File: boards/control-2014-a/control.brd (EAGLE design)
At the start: 285 parts, among them J1 0528520870, J10 2MM-6H, J11 JST_VH_2, J12 2MM-4V, J13 2MM-4H, J14 2MM-4H, J15 2MM-4H, J16 2MM-4H, J17 2MM-8H, J19 JST_VH_2, J2 MINI-USB, J20 2MM-5V, J3 2MM-2H, J4 Molex 0522711179, J5 Molex 0522711179, J6 Molex 0522711179, J7 Molex 0522711179, J8 MMCX_RA, J9 2MM-3H, Q1 IRF9310TRPBF, Q10 IRF8734TRPBF, Q11 IRF9310TRPBF, Q12 IRF8734TRPBF, Q13 IRF9310TRPBF, Q14 IRF8734TRPBF, Q15 IRF9310TRPBF, Q16 IRF8734TRPBF, Q17 IRF9310TRPBF, Q18 IRF8734TRPBF, Q19 IRF9310TRPBF, Q2 IRF8734TRPBF, Q20 IRF8734TRPBF, Q21 IRF9310TRPBF, Q22 IRF8734TRPBF, Q23 IRF9310TRPBF, Q24 IRF8734TRPBF, Q25 IRF9310TRPBF, Q26 IRF8734TRPBF, Q27 IRF9310TRPBF, Q28 IRF8734TRPBF, Q29 IRF9310TRPBF, Q3 IRF9310TRPBF, Q30 IRF8734TRPBF, Q33 FDV304P, Q4 IRF8734TRPBF, Q5 IRF9310TRPBF, Q6 IRF8734TRPBF, Q7 IRF9310TRPBF, Q8 IRF8734TRPBF, Q9 IRF9310TRPBF, U1 XC3S100E, U10 CC1101, U12 TC4428, U13 0896BM15A0001, U15 TC4428, U18 TC4428, U19 IMU3000, U2 M25P10, U20 KXTF9-2050, U21 TC4428, U24 TC4428, U27 TC4428, U3 LM2734, U30 TC4428, U33 TC4428, U36 TC4428, U39 TC4428, U4 MCP1824T-1202E/OT, U42 TC4428, U45 TC4428, U48 TC4428, U5 MCP1824T-2502E/OT, U6 TC4428, U7 AT91SAM7S256, U8 MCP1824ST-3302E/DB, U9 TC4428, X1 18.432MHz, X2 644-1055-1-ND

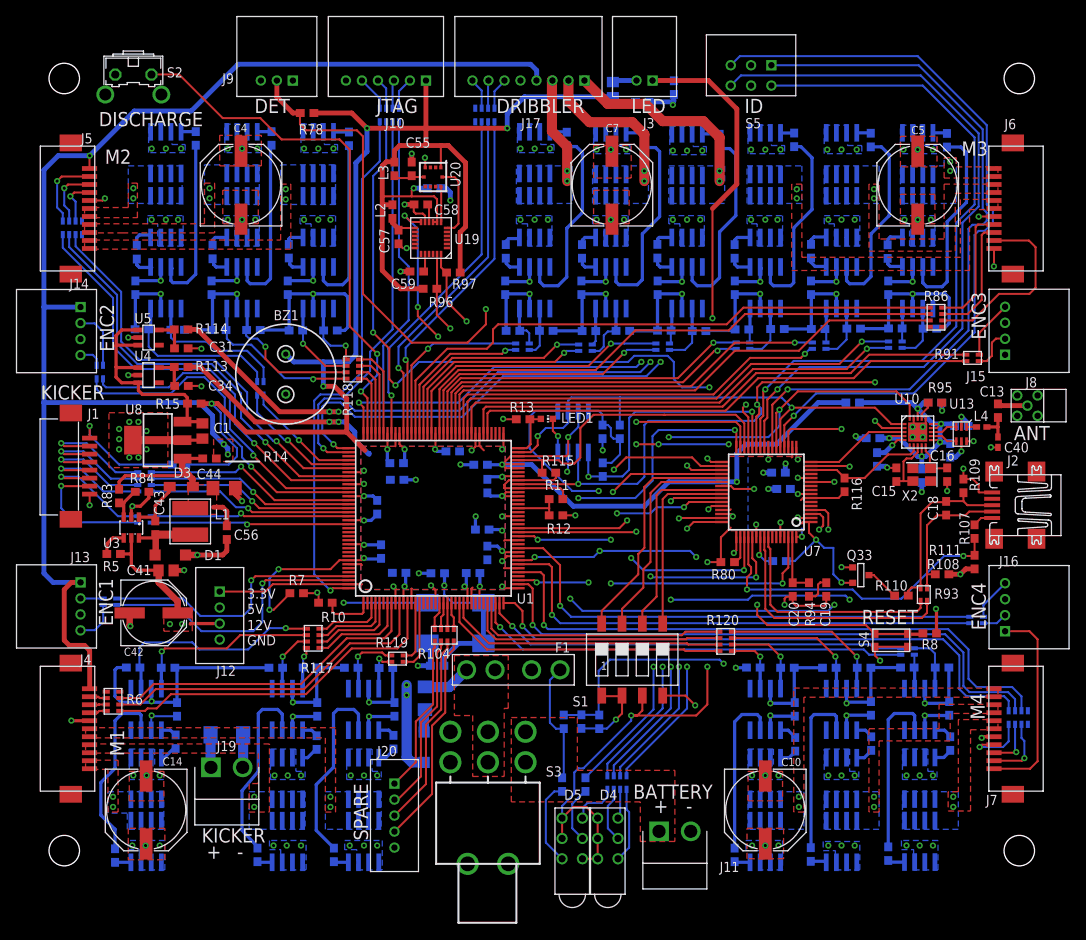
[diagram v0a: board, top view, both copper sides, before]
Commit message: control-2014-a
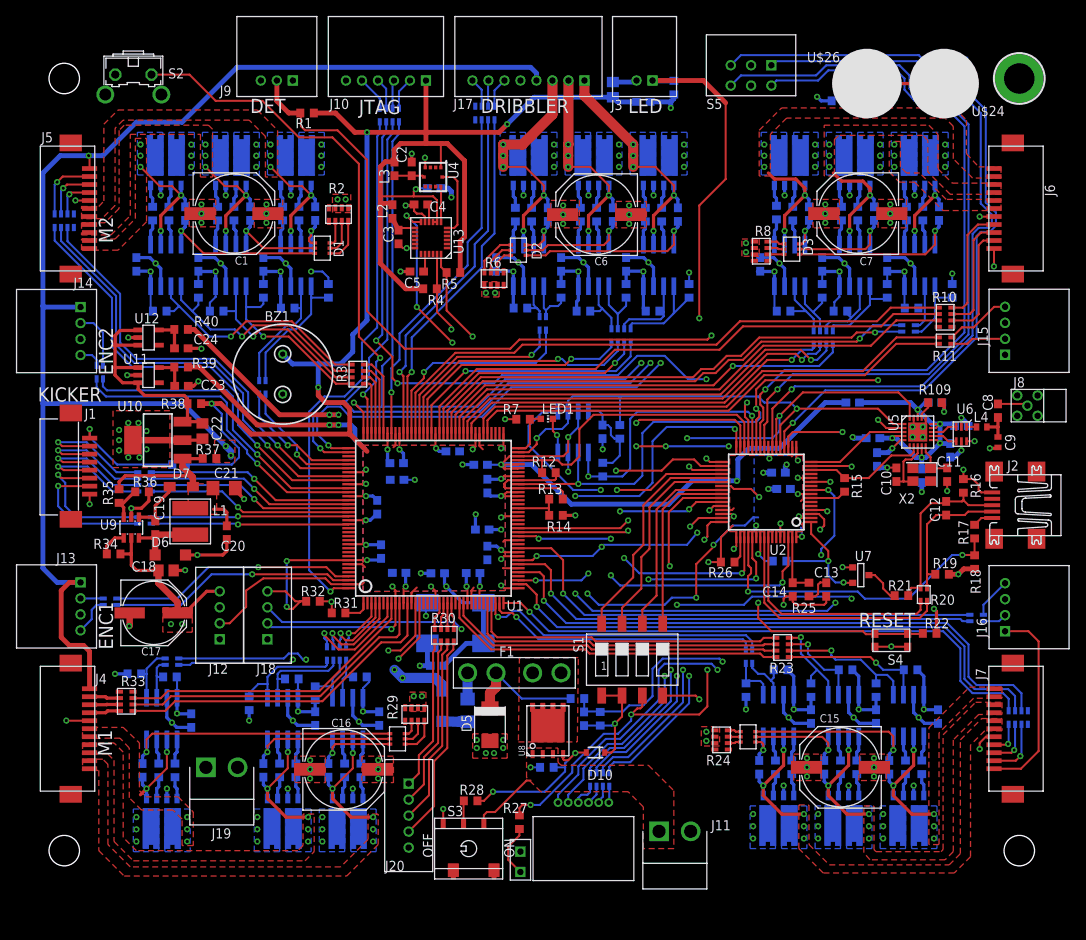
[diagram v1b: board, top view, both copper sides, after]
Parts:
- removed Q33: FDV304P, zetex:SOT-23
- removed R131: 220, resistor-array:RA_2_0606
- removed U15, U18, U21, U24, U27, U30, U33, U36, U39, U42, U45, U48: TC4428, microchip:SO08
- removed U19: IMU3000, inertial-sensors:IMU3000
- removed U20: KXTF9-2050, inertial-sensors:KXTF9
- added C45, C69, C75: 47nF, rcl:C0603
- added C61, C63, C64, C65, C66, C70, C72, C73, C74, C76, C78: 100nF, rcl:C0603
- added C62: 10nF, rcl:C0603
- added D10: CDSOD323-T15SC, CDSOD323-TxxSC:SOD-323
- added D7: BAS16H, diode:SOD323-W
- added D8: MMBD4448HTW, Diode-Array:MMBD4448HTW
- added D9: MBRX160-TP, diode:SOD123
- added H1: (no value), Mounting_Hole:MOUNTING_HOLE
- added J18: 2MM-4V, 2mm:2MM-4-V
- added LED2: LED2, 5350T5:5350T5
- added LED3: LDS-M514RI-RA, rjrc-7seg-disp:LDS-M514RI-RA
- added R100: 220, resistor-array:RA_2_0606
- added R101, R121: 10.0k, rcl:R0603
- added R106, R126: 220, resistor-array:RA_4_1206
- added R127: 0, rcl:R0603
- added R98, R99: 22, rcl:R0603
- added U$24, U$26: RL1014, RLB1014-inductor:RL1014
- added U11: MCP1824T-1202E/OT, power:SOT23-5
- C1: value 10uF -> 470uF 25V; device rcl:C0805 -> rcl:PANASONIC_G
- C10: value 470uF 25V -> 27pF; device rcl:PANASONIC_G -> rcl:C0603
- C11: value 10nF -> 27pF
- C12: value 220nF -> 33pF
- C13: value 100pF -> 10nF
- C14: value 470uF 25V -> 1nF; device rcl:PANASONIC_G -> rcl:C0603
- C15, C16: value 27pF -> 470uF 25V; device rcl:C0603 -> rcl:PANASONIC_G
- C17: value 100nF -> 100uF 25V; device rcl:C0603 -> rcl:PANASONIC_E
- C18: value 33pF -> 1uF 35V; device rcl:C0603 -> rcl:C0805
- C20: value 1nF -> 100nF
- C21: value 100nF -> 22uF 6.3V; device rcl:C0603 -> rcl:C1206
- C22: value 100nF -> 10uF; device rcl:C0603 -> rcl:C0805
- C23, C24, C50: value 100nF -> 1uF
- C3, C31, C34: value 1uF -> 100nF
- C38, C47, C49, C52, C54, C56, C67, C71, C77, C79: value 100nF -> 47nF
- C4: value 470uF 25V -> 100nF; device rcl:PANASONIC_G -> rcl:C0603
- C40: value 500R07S1R8BV4T -> 47nF; device rcl:C0402 -> rcl:C0603
- C41: value 1uF 35V -> 100nF; device rcl:C0805 -> rcl:C0603
- C42: value 100uF 25V -> 47nF; device rcl:PANASONIC_E -> rcl:C0603
- C43: value 10nF -> 100nF
- C44: value 22uF 6.3V -> 100nF; device rcl:C1206 -> rcl:C0603
- C5: value 470uF 25V -> 2.2nF; device rcl:PANASONIC_G -> rcl:C0603
- C57: value 100nF -> 220nF
- C6: value 100nF -> 470uF 25V; device rcl:C0603 -> rcl:PANASONIC_G
- C60: value 100nF -> 10nF
- C8: value 10nF -> 100pF
- C9: value 2.2nF -> 500R07S1R8BV4T; device rcl:C0603 -> rcl:C0402
- D1, D2: value MBRX160-TP -> MMBD4448HTW; device diode:SOD123 -> Diode-Array:MMBD4448HTW
- D3: value BAS16H -> MMBD4448HTW; device diode:SOD323-W -> Diode-Array:MMBD4448HTW
- D4: value 564-0100-132F -> MMBD4448HTW; device led-array:DIALIGHT-564 -> Diode-Array:MMBD4448HTW
- D5: value 564-0100-132F -> SMBJP6KE18A-TP; device led-array:DIALIGHT-564 -> power:SMBJ
- D6: value SMBJP6KE18A-TP -> MBRX160-TP; device power:SMBJ -> diode:SOD123
- F1: value 2x BK6011 -> 2x BK6011 [30A]
- J11: value JST_VH_2 -> BATT
- Q1, Q11, Q13, Q15, Q17, Q19, Q21, Q23, Q25, Q27, Q29, Q3, Q5, Q7, Q9: value IRF9310TRPBF -> FAN7380; device onsemi:SO8 -> microchip:SO08
- Q10, Q12, Q14, Q16, Q18, Q2, Q20, Q22, Q24, Q26, Q28, Q30, Q4, Q6, Q8: value IRF8734TRPBF -> BSC072N03LD; device onsemi:SO8 -> Dual N-Channel MOSFET:BSC072N03LD
- R1: value 220 -> 5.6k; device resistor-array:RA_4_1206 -> rcl:R0603
- R10: device rcl:R0603 -> resistor-array:RA_4_1206
- R102, R14, R15: value 0 -> 10.0k
- R103, R122, R123: value 220 -> 22; device resistor-array:RA_2_0606 -> rcl:R0603
- R104, R117, R118, R85, R86: value 220 -> 22; device resistor-array:RA_4_1206 -> rcl:R0603
- R105: value NP -> 100k
- R107, R79: value 220 -> 10.0k
- R108: value 330k -> 68k
- R109: value 330k -> 56k
- R11: value NP -> 220; device rcl:R0603 -> resistor-array:RA_2_0606
- R110: value 1.5k -> 220; device rcl:R0603 -> resistor-array:RA_4_1206
- R113, R114: value 0 -> 22
- R115: value NP -> 10.0k
- R12: value 10.0k -> NP
- R120, R4, R87, R88: value 220 -> 10.0k; device resistor-array:RA_4_1206 -> rcl:R0603
- R129, R130: value 220 -> 10K; device resistor-array:RA_2_0606 -> rcl:R0603
- R13: value 220 -> NP
- R16: value 100k -> 330k
- R17: value 1.5k -> 220
- R18, R22, R34, R42, R43, R46, R47, R50, R51, R58, R59, R63, R67, R74, R75: value 10 -> 10.0k
- R19: value 10 -> 330k
- R2, R24, R29, R8: value 10.0k -> 22; device rcl:R0603 -> resistor-array:RA_4_1206
- R20: value 10.0k -> 27; device rcl:R0603 -> resistor-array:RA_2_0606
- R21, R25: value 10.0k -> 1.5k
- R23, R30, R55, R62: value 10 -> 220; device rcl:R0603 -> resistor-array:RA_4_1206
- R26: value 10 -> NP
- R27, R31: value 10 -> 220
- R28: value 10.0k -> 10
- R33, R41, R56, R73: value 10.0k -> 220; device rcl:R0603 -> resistor-array:RA_4_1206
- R35: value 10 -> 52.3k
- R37, R40: value 10.0k -> 0
- R38, R39: value 10 -> 0
- R44, R45, R48, R49, R52, R53, R60, R61, R65, R69, R76, R77: value 10.0k -> 22
- R54: value 10 -> 220; device rcl:R0603 -> resistor-array:RA_2_0606
- R57, R82: value 10.0k -> 220; device rcl:R0603 -> resistor-array:RA_2_0606
- R6: value 220 -> 22
- R66, R70: value 10 -> 22
- R7: value 10.0k -> 220
- R71: value 10 -> 150 1/8W; device rcl:R0603 -> rcl:R0805
- R72: value 10.0k -> 100k
- R78: value 5.6k -> 10.0k
- R80: value NP -> 22
- R81: value 68k -> 22
- R83: value 52.3k -> 10.0k
- R89: value 220 -> NP; device resistor-array:RA_2_0606 -> rcl:R0603
- R9: value 150 1/8W -> 10K; device rcl:R0805 -> rcl:R0603
- R91: device resistor-array:RA_2_0606 -> resistor-array:RA_4_1206
- R92: value 220 -> 10.0k; device resistor-array:RA_2_0606 -> rcl:R0603
- R93: value 27 -> 10.0k; device resistor-array:RA_2_0606 -> rcl:R0603
- R94: value 1.5k -> 22
- R95: value 56k -> 22
- S3: value M2022S2A2W30 -> G3T12AP_SPDT; device switch-robocup:M202X-30 -> switch-robocup:G3T12AP_SP
- U10: value CC1101 -> MCP1824ST-3302E/DB; device radio:QLP20 -> power:SOT223
- U12: value TC4428 -> MCP1824T-2502E/OT; device microchip:SO08 -> power:SOT23-5
- U13: value 0896BM15A0001 -> IMU3000; device radio:0896BM15A0001 -> inertial-sensors:IMU3000
- U2: value M25P10 -> AT91SAM7S256; device st_micro:SO08 -> at91sam7:SQFP-S-10X10-64
- U3: value LM2734 -> M25P10; device power:SOT23-6L -> st_micro:SO08
- U4: value MCP1824T-1202E/OT -> KXTF9-2050; device power:SOT23-5 -> inertial-sensors:KXTF9
- U5: value MCP1824T-2502E/OT -> CC1101; device power:SOT23-5 -> radio:QLP20
- U6: value TC4428 -> 0896BM15A0001; device microchip:SO08 -> radio:0896BM15A0001
- U7: value AT91SAM7S256 -> FDV304P; device at91sam7:SQFP-S-10X10-64 -> zetex:SOT-23
- U8: value MCP1824ST-3302E/DB -> SI7141DP; device power:SOT223 -> rjrc_power_transistors:POWERPAK_SO-8
- U9: value TC4428 -> LM2734; device microchip:SO08 -> power:SOT23-6L
- moved Q8 121.7 mm to (12.7, 86.0), turned to 90 degrees
- moved Q6 121.0 mm to (12.2, 3.68), turned to 270 degrees
- moved R90 113.8 mm to (114.0, 29.1), turned to 90 degrees
- moved Q24 107.3 mm to (89.3, 4.06), turned to 270 degrees
- moved R128 106.8 mm to (4.45, 59.8), turned to 0 degrees
- moved R123 106.3 mm to (11.8, 10.0), turned to 270 degrees
- moved R22 105.5 mm to (108.2, 27.2), flipped to the top, turned to 0 degrees
- moved R55 105.3 mm to (40.6, 91.9), turned to 0 degrees
- moved R84 104.3 mm to (111.0, 70.0), flipped to the bottom, turned to 270 degrees
- moved R85 104.3 mm to (105.3, 79.6), turned to 90 degrees
- moved Q23 104.0 mm to (89.3, 16.9)
- moved R83 101.8 mm to (105.9, 67.8), flipped to the bottom, turned to 180 degrees
- moved R42 100.7 mm to (11.9, 67.4), turned to 180 degrees
- moved R44 98.2 mm to (11.0, 79.6), turned to 90 degrees
- moved C18 97.8 mm to (12.7, 35.0), turned to 0 degrees
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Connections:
- removed net LED_LR: R1.8, U7.35
- removed net LED_LY: R79.1, U7.42
- removed net LED_RG: R1.2, U7.48
- removed net LED_RR: R1.4, U7.47
- removed net LED_RY: R1.6, U7.15
- new net CHASSIS: H1.GND, R9.1, U$24.P$1
- new net LED_AE: R106.8, U2.35
- new net LED_AN1: LED3.1, U2.9
- new net LED_AN2: LED3.2, U2.42
- new net LED_BF: R106.6, U2.15
- new net LED_CG: R106.4, U2.47
- new net LED_DDP: R106.2, U2.48
- new net N$100: Q17.7, R86.1
- new net N$174: Q11.2, R62.4, R67.2
- new net N$175: Q11.7, R70.1
- new net N$176: D2.A2, R6.5
- new net N$177: Q26.G1, R70.2
- new net N$178: Q11.5, R69.1
- new net N$179: Q26.G2, R69.2
- new net N$180: Q11.1, R62.2, R68.2
- new net N$181: Q9.2, R62.8, R63.2
- new net N$182: Q9.7, R66.1
- new net N$183: Q28.G1, R66.2
- new net N$184: Q9.5, R65.1
- new net N$185: Q28.G2, R65.2
- new net N$186: Q9.1, R62.6, R64.2
- new net N$187: Q7.2, R57.4, R58.2
- new net N$188: Q7.7, R61.1
- new net N$189: Q30.G1, R61.2
- new net N$190: Q7.5, R60.1
- new net N$191: Q30.G2, R60.2
- new net N$192: Q7.1, R57.2, R59.2
- new net N$193: C49.1, D2.C3, Q11.8
- new net N$194: C47.1, D2.C2, Q9.8
- new net N$195: C45.1, D2.C1, Q7.8
- new net N$196: D2.A1, R6.7
- new net N$197: D2.A3, R6.3
- new net N$198: R28.1, S3.5
- new net N$199: D10.2, R105.1, R28.2, U8.4
- new net N$200: R130.2, U$24.P$2, U$26.P$1
- new net N$201: R129.1, U$26.P$2
- new net N$3: Q25.2, R110.8, R111.2
- new net N$94: F1.1, F1.2, U8.D@1, U8.D@2, U8.D@3, U8.D@4
- new net N$95: Q15.1, R73.2, R79.2
- new net VBATT: J11.1, R105.2, S3.4, U8.S@1, U8.S@2, U8.S@3
- net +1.2V: now also C26.1, C27.1, C31.1, C34.1, J18.2, R39.1; no longer C24.1, C50.1, C51.1, C71.1, R113.1
- net +1.8V: now also C64.1, J18.3, U2.12, U2.24, U2.54, U2.64, U2.8; no longer C79.1, U7.12, U7.24, U7.54, U7.64, U7.8
- net +12V: now also C1.+, C15.+, C16.+, C41.1, C44.1, C46.1, C48.1, C51.1, C53.1, C55.1, C6.+, C66.1, C68.1, C70.1, C74.1, C76.1, C78.1, D5.C, F2.1, Q10.D1@1, Q10.D1@2, Q12.D1@1, Q12.D1@2, Q14.D1@1, Q14.D1@2, Q16.D1@1, Q16.D1@2, Q18.D1@1, Q18.D1@2, Q2.D1@1, Q2.D1@2, Q20.D1@1, Q20.D1@2, Q22.D1@1, Q22.D1@2, Q24.D1@1, Q24.D1@2, Q26.D1@1, Q26.D1@2, Q28.D1@1, Q28.D1@2, Q30.D1@1, Q30.D1@2, Q4.D1@1, Q4.D1@2, Q6.D1@1, Q6.D1@2, Q8.D1@1, Q8.D1@2, R108.2, R2.4, R2.6, R2.8, R24.4, R24.6, R24.8, R29.4, R29.6, R29.8, R6.4, R6.6, R6.8, R8.4, R8.6, R8.8; no longer C10.+, C14.+, C2.1, C21.1, C22.1, C26.1, C27.1, C28.1, C29.1, C30.1, C32.1, C33.1, C35.1, C36.1, C38.1, C4.+, C5.+, D6.C, Q1.1, Q1.2, Q11.1, Q11.2, Q13.1, Q13.2, Q15.1, Q15.2, Q17.1, Q17.2, Q19.1, Q19.2, Q21.1, Q21.2, Q23.1, Q23.2, Q25.1, Q25.2, Q27.1, Q27.2, Q29.1, Q29.2, Q3.1, Q3.2, Q5.1, Q5.2, Q7.1, Q7.2, Q9.1, Q9.2, R17.2, R81.2, U12.6, U15.6, U18.6, U21.6, U24.6, U27.6, U30.6, U33.6, U36.6, U39.6, U42.6, U45.6, U48.6, U6.6, U9.6
- net +2.5V: now also C25.1, C29.1, C32.1, C35.1, J18.4, R32.1, R40.1; no longer C23.1, C49.1, C67.1, C68.1, R114.1, R13.1
- net +3.3V: now also C28.1, C30.1, C33.1, C36.1, C43.1, C50.1, C63.1, C65.1, C73.1, J12.2, R1.1, R12.2, R127.1, R13.2, R22.2, R26.2, R27.2, R38.2, R4.2, R5.2, R71.1, R87.2, R88.2, R89.2, U13.8, U13.9, U2.1, U2.18, U2.45, U2.58, U2.59, U3.3, U3.7, U3.8, U4.1, U7.2; no longer C3.1, C46.1, C47.1, C48.1, C52.1, C53.1, C54.1, C60.1, C77.1, D4.A1, D4.A2, D4.A3, D5.A1, D5.A2, D5.C3, J12.1, Q33.2, R102.1, R105.2, R11.2, R112.2, R115.2, R116.2, R2.2, R78.1, R8.2, R80.2, R9.1, R96.2, R97.2, U19.8, U19.9, U2.3, U2.8, U20.1, U7.1, U7.18, U7.45, U7.58, U7.59, U7.7
- net +5V: now also J12.3, R37.2; no longer J12.2, R14.2
- net /CONNECT: now also U2.19, U7.3; no longer Q33.3, U7.19
- net 12V_LOGIC: now also C17.+, C18.1, D9.C, J12.4, R34.2, U9.5; no longer C41.1, C42.+, D2.C, J12.3, R5.2, U3.5
- net ARM_TDI: now also U2.33; no longer U7.33
- net ARM_TDO: now also R55.5, U2.49; no longer R3.5, U7.49
- net BALL_DET: now also R1.2, U2.3; no longer R78.2, U7.3
- net BALL_LED: now also R72.1, U2.44; no longer R16.1, U7.44
- net BATT_SENSE: now also C72.1, R107.2, R108.1, U2.4; no longer C25.1, R81.1, R82.2, U7.4
- net BUZZ: now also U2.32; no longer U7.32
- net DDM: now also R20.2, U2.56; no longer R93.2, U7.56
- net DDP: now also R20.4, U2.57; no longer R93.4, U7.57
- net DONE: now also R7.2; no longer R13.2
- net DP1: now also U2.37; no longer U7.37
- net DP2: now also U2.38; no longer U7.38
- net DP4: now also U2.41; no longer U7.41
- net FLASH_NCS: now also R88.1, U2.28, U3.1; no longer R112.1, U2.1, U7.28
- net FPGA_NCS: now also R12.1, U2.30; no longer R115.1, U7.30
- net FPGA_SPARE_0: now also R30.2; no longer R104.2
- net FPGA_SPARE_1: now also R30.4; no longer R104.4
- net FPGA_SPARE_2: now also R30.6; no longer R104.6
- net FPGA_SPARE_3: now also R30.8; no longer R104.8
- net FPGA_TDI: now also R55.7; no longer R3.7
- net FS0: now also U2.31; no longer U7.31
- net FS1: now also U2.29; no longer U7.29
- net GND: now also C1.-, C10.2, C13.2, C14.2, C15.-, C16.-, C17.-, C18.2, C4.2, C43.2, C5.2, C6.-, C61.2, C62.2, C63.2, C64.2, C65.2, C66.2, C70.2, C72.2, C73.2, C74.2, C76.2, C78.2, D10.1, D5.A, J12.1, J18.1, J9.3, LED2.CATHODE, Q1.4, Q10.S2, Q11.4, Q12.S2, Q13.4, Q14.S2, Q15.4, Q16.S2, Q17.4, Q18.S2, Q19.4, Q2.S2, Q20.S2, Q21.4, Q22.S2, Q23.4, Q24.S2, Q25.4, Q26.S2, Q27.4, Q28.S2, Q29.4, Q3.4, Q30.S2, Q4.S2, Q5.4, Q6.S2, Q7.4, Q8.S2, Q9.4, R101.1, R102.1, R107.1, R112.1, R115.1, R116.1, R120.1, R121.1, R129.2, R130.1, R14.1, R16.1, R18.1, R19.1, R42.1, R43.1, R46.1, R47.1, R50.1, R51.1, R58.1, R59.1, R63.1, R67.1, R72.2, R74.1, R75.1, R78.1, R79.1, R83.1, R9.2, R92.1, R93.1, R96.1, R97.1, S3.6, U10.2, U10.4, U11.2, U12.2, U13.11, U13.18, U2.17, U2.2, U2.46, U2.60, U3.4, U4.4, U5.16, U5.19, U5.DAP, U6.2, U6.5, U6.6, U9.2; no longer C1.2, C10.-, C12.2, C14.-, C15.2, C16.2, C17.2, C19.2, C38.2, C4.-, C40.2, C42.-, C47.2, C49.2, C5.-, C52.2, C54.2, C56.2, C6.2, C67.2, C71.2, C77.2, C79.2, C8.2, D1.A, J12.4, Q10.1, Q10.2, Q10.3, Q12.1, Q12.2, Q12.3, Q14.1, Q14.2, Q14.3, Q16.1, Q16.2, Q16.3, Q18.1, Q18.2, Q18.3, Q2.1, Q2.2, Q2.3, Q20.1, Q20.2, Q20.3, Q22.1, Q22.2, Q22.3, Q24.1, Q24.2, Q24.3, Q26.1, Q26.2, Q26.3, Q28.1, Q28.2, Q28.3, Q30.1, Q30.2, Q30.3, Q4.1, Q4.2, Q4.3, Q6.1, Q6.2, Q6.3, Q8.1, Q8.2, Q8.3, R108.1, R12.1, R16.2, R20.1, R21.1, R24.1, R25.1, R28.1, R29.1, R32.1, R33.1, R37.1, R40.1, R41.1, R44.1, R45.1, R48.1, R49.1, R52.1, R53.1, R56.1, R57.1, R60.1, R61.1, R65.1, R69.1, R72.1, R73.1, R76.1, R77.1, R82.1, R95.1, U10.16, U10.19, U10.DAP, U12.3, U13.2, U13.5, U13.6, U15.3, U18.3, U19.11, U19.18, U2.4, U20.4, U21.3, U24.3, U27.3, U3.2, U30.3, U33.3, U36.3, U39.3, U4.2, U42.3, U45.3, U48.3, U5.2, U6.3, U7.17, U7.2, U7.46, U7.60, U8.2, U8.4, U9.3
- net I2C_SCL: now also R4.1, U13.23, U2.36; no longer R96.1, U19.23, U7.36
- net I2C_SDA: now also R5.1, U13.24, U2.43; no longer R97.1, U19.24, U7.43
- net ID0: now also U2.23; no longer U7.23
- net ID1: now also U2.25; no longer U7.25
- net ID2: now also U2.20; no longer U7.20
- net ID3: now also U2.26; no longer U7.26
- net IMU_INT: now also U13.12, U2.34; no longer U19.12, U7.34
- net KCHARGE: now also R126.2; no longer R4.2
- net KCHIP: now also R125.3; no longer R103.3
- net KDONE: now also R126.4; no longer R4.4
- net KKICK: now also R125.1; no longer R103.1
- net KSCL: now also R126.6; no longer R4.6
- net KSDA: now also R126.8; no longer R4.8
- net M1A: now also C75.2, Q2.D2@1, Q2.D2@2, Q2.S1, Q25.6; no longer Q11.5, Q11.6, Q11.7, Q11.8, Q12.5, Q12.6, Q12.7, Q12.8
- net M1A_H: now also R110.7; no longer R117.7
- net M1A_L: now also R110.5; no longer R117.5
- net M1B: now also C77.2, Q27.6, Q4.D2@1, Q4.D2@2, Q4.S1; no longer Q1.5, Q1.6, Q1.7, Q1.8, Q2.5, Q2.6, Q2.7, Q2.8
- net M1B_H: now also R110.3; no longer R117.3
- net M1B_L: now also R110.1; no longer R117.1
- net M1C: now also C79.2, Q29.6, Q6.D2@1, Q6.D2@2, Q6.S1; no longer Q21.5, Q21.6, Q21.7, Q21.8, Q22.5, Q22.6, Q22.7, Q22.8
- net M1ENC_A: now also R124.1; no longer R89.1
- net M1ENC_B: now also R124.3; no longer R89.3
- net M1HALL_A: now also R33.3; no longer R6.3
- net M1HALL_B: now also R33.1; no longer R6.1
- net M1HALL_C: now also R33.5; no longer R6.5
- net M2: now also R13.1, R14.2; no longer R11.1, R12.2
- net M2A: now also C38.2, Q1.6, Q8.D2@1, Q8.D2@2, Q8.S1; no longer Q3.5, Q3.6, Q3.7, Q3.8, Q4.5, Q4.6, Q4.7, Q4.8
- net M2A_H: now also R3.7; no longer R118.7
- net M2A_L: now also R3.5; no longer R118.5
- net M2B: now also C40.2, Q10.D2@1, Q10.D2@2, Q10.S1, Q3.6; no longer Q13.5, Q13.6, Q13.7, Q13.8, Q14.5, Q14.6, Q14.7, Q14.8
- net M2B_H: now also R3.3; no longer R118.3
- net M2B_L: now also R3.1; no longer R118.1
- net M2C: now also C42.2, Q12.D2@1, Q12.D2@2, Q12.S1, Q5.6; no longer Q23.5, Q23.6, Q23.7, Q23.8, Q24.5, Q24.6, Q24.7, Q24.8
- net M2C_H: now also R54.3; no longer R122.1
- net M2C_L: now also R54.1; no longer R122.3
- net M2ENC_A: now also R128.1; no longer R90.1
- net M2ENC_B: now also R128.3; no longer R90.3
- net M2HALL_A: now also R41.5; no longer R85.5
- net M2HALL_B: now also R41.3; no longer R85.3
- net M2HALL_C: now also R41.7; no longer R85.7
- net M3A: now also C52.2, Q13.6, Q14.D2@1, Q14.D2@2, Q14.S1; no longer Q5.5, Q5.6, Q5.7, Q5.8, Q6.5, Q6.6, Q6.7, Q6.8
- net M3A_H: now also R73.7; no longer R123.1
- net M3A_L: now also R73.5; no longer R123.3
- net M3B: now also C54.2, Q16.D2@1, Q16.D2@2, Q16.S1; no longer Q15.5, Q15.7, Q15.8, Q16.5, Q16.6, Q16.7, Q16.8
- net M3B_H: now also R73.3; no longer R124.1
- net M3B_L: now also R73.1; no longer R124.3
- net M3C: now also C56.2, Q17.6, Q18.D2@1, Q18.D2@2, Q18.S1; no longer Q25.5, Q25.6, Q25.7, Q25.8, Q26.5, Q26.6, Q26.7, Q26.8
- net M3C_H: now also R82.3; no longer R125.1
- net M3C_L: now also R82.1; no longer R125.3
- net M3ENC_A: now also R11.2; no longer R91.2
- net M3ENC_B: now also R11.4; no longer R91.4
- net M3HALL_A: now also R10.3; no longer R86.3
- net M3HALL_B: now also R10.1; no longer R86.1
- net M3HALL_C: now also R10.5; no longer R86.5
- net M4A: now also C67.2, Q19.6, Q20.D2@1, Q20.D2@2, Q20.S1; no longer Q27.5, Q27.6, Q27.7, Q27.8, Q28.5, Q28.6, Q28.7, Q28.8
- net M4A_H: now also R23.7; no longer R120.7
- net M4A_L: now also R23.5; no longer R120.5
- net M4B: now also C69.2, Q21.6, Q22.D2@1, Q22.D2@2, Q22.S1; no longer Q17.5, Q17.6, Q17.7, Q17.8, Q18.5, Q18.6, Q18.7, Q18.8
- net M4B_H: now also R23.3; no longer R120.3
- net M4B_L: now also R23.1; no longer R120.1
- net M4C: now also C71.2, Q23.6, Q24.D2@1, Q24.D2@2, Q24.S1; no longer Q7.5, Q7.6, Q7.7, Q7.8, Q8.5, Q8.6, Q8.7, Q8.8
- net M4C_H: now also R100.3; no longer R128.1
- net M4C_L: now also R100.1; no longer R128.3
- net M4ENC_A: now also R90.1; no longer R92.1
- net M4ENC_B: now also R90.3; no longer R92.3
- net M4HALL_A: now also R91.3; no longer R87.3
- net M4HALL_B: now also R91.1; no longer R87.1
- net M4HALL_C: now also R91.5; no longer R87.5
- net M5A: now also C49.2, Q11.6, Q26.D2@1, Q26.D2@2, Q26.S1; no longer Q10.5, Q10.6, Q10.7, Q10.8, Q9.5, Q9.6, Q9.7, Q9.8
- net M5A_H: now also R62.3; no longer R129.1
- net M5A_L: now also R62.1; no longer R129.3
- net M5B: now also C47.2, Q28.D2@1, Q28.D2@2, Q28.S1, Q9.6; no longer Q19.5, Q19.6, Q19.7, Q19.8, Q20.5, Q20.6, Q20.7, Q20.8
- net M5B_H: now also R62.7; no longer R130.1
- net M5B_L: now also R62.5; no longer R130.3
- net M5C: now also C45.2, Q30.D2@1, Q30.D2@2, Q30.S1, Q7.6; no longer Q29.5, Q29.6, Q29.7, Q29.8, Q30.5, Q30.6, Q30.7, Q30.8
- net M5C_H: now also R57.3; no longer R131.1
- net M5C_L: now also R57.1; no longer R131.3
- net M5HALL_A: now also R56.1; no longer R88.1
- net M5HALL_B: now also R56.3; no longer R88.3
- net M5HALL_C: now also R56.5; no longer R88.5
- net MCU_PROGB: now also R31.1, R32.2, U2.11; no longer R10.1, R7.2, U7.11
- net MISO: now also U2.27, U3.2, U5.2; no longer U10.2, U2.2, U7.27
- net MOSI: now also U2.22, U3.5, U5.20; no longer U10.20, U2.5, U7.22
- net N$1: now also R124.4; no longer R89.4
- net N$10: now also LED3.4, R106.5; no longer Q6.4, R43.1
- net N$101: now also U13.7, U4.9; no longer U19.7, U20.9
- net N$102: now also C19.1, D7.C, U9.1; no longer C43.1, D3.C, U3.1
- net N$103: now also Q18.G1, R86.2; no longer F1.1, F1.2, F2.1, S3.2, S3.5
- net N$104: now also R126.1; no longer R4.1
- net N$105: now also R35.1, R36.2, U9.3; no longer R83.1, R84.2, U3.3
- net N$106: now also R55.6; no longer R3.6
- net N$107: now also R89.1, U2.55; no longer R105.1, U7.55
- net N$108: now also R55.2; no longer R3.2
- net N$109: now also C12.1, R16.2, R20.3, R21.1; no longer C18.1, R109.2, R110.1, R93.3
- net N$11: now also C20.1, C21.1, D7.A, R35.2, R37.1, U10.1; no longer C44.1, C56.1, D3.A, R14.1, R83.2, U8.1
- net N$110: now also R21.2, U7.1; no longer Q33.1, R110.2
- net N$111: now also C13.1, R25.1; no longer C19.1, R94.1
- net N$112: now also C14.1, R25.2, U2.63; no longer C20.1, R94.2, U7.63
- net N$113: now also Q17.5, R85.1; no longer D4.C1, R1.3
- net N$114: now also D9.A; no longer D2.A
- net N$115: now also Q18.G2, R85.2; no longer D5.C1, R1.7
- net N$116: now also Q17.1, R82.2, R84.2; no longer D5.C2, R79.2
- net N$117: now also R124.2; no longer R89.2
- net N$118: now also R90.4; no longer R92.4
- net N$119: now also R90.2; no longer R92.2
- net N$12: now also LED3.3, R106.7; no longer Q8.4, R55.1
- net N$120: now also R11.3; no longer R91.3
- net N$121: now also R11.1; no longer R91.1
- net N$122: now also R128.4; no longer R90.4
- net N$123: now also R128.2; no longer R90.2
- net N$124: now also C52.1, D3.C1, Q13.8; no longer D5.A3, R17.1
- net N$125: now also U13.6, U4.10; no longer U19.6, U20.10
- net N$126: now also C3.1, U13.13; no longer C57.1, U19.13
- net N$127: now also C4.1, U13.10; no longer C58.1, U19.10
- net N$128: now also C5.1, U13.20; no longer C59.1, U19.20
- net N$129: now also R125.2; no longer R103.2
- net N$13: now also LED2.ANODE, R27.1; no longer Q11.4, R22.1
- net N$130: now also R125.4; no longer R103.4
- net N$131: now also R127.2; no longer R102.2
- net N$132: now also C61.1, U5.5; no longer C17.1, U10.5
- net N$133: now also R109.2, U5.17; no longer R95.2, U10.17
- net N$134: now also C11.1, U5.10; no longer C16.1, U10.10
- net N$135: now also R30.5; no longer R104.5
- net N$136: now also R30.3; no longer R104.3
- net N$137: now also R30.1; no longer R104.1
- net N$138: now also R30.7; no longer R104.7
- net N$139: now also C10.1, U5.8; no longer C15.1, U10.8
- net N$14: now also Q2.G2, R113.2; no longer R19.2, U6.5
- net N$140: now also C54.1, D3.C2, Q15.8; no longer R117.2, R21.2, U6.4
- net N$141: now also U6.1; no longer U13.1
- net N$142: now also C56.1, D3.C3, Q17.8; no longer R117.4, R20.2, U6.2
- net N$143: now also C8.1, C9.1; no longer C13.1, C40.1
- net N$144: now also R17.2; no longer R107.2
- net N$145: now also U5.12, U6.4; no longer U10.12, U13.4
- net N$146: now also D3.A1, R8.7; no longer R119.2, R29.2, U12.4
- net N$147: now also D3.A3, R8.3; no longer R119.4, R28.2, U12.2
- net N$148: now also Q19.2, R23.8, R92.2; no longer R122.2, R40.2, U21.2
- net N$149: now also Q19.7, R95.1; no longer R122.4, R41.2, U21.4
- net N$15: now also Q25.1, R110.6, R112.2; no longer Q12.4, R23.1
- net N$150: now also D4.A2, R24.5; no longer R118.4, R36.2, U18.2
- net N$151: now also Q20.G1, R95.2; no longer R118.2, R37.2, U18.4
- net N$152: now also Q19.5, R94.1; no longer R118.8, R32.2, U15.2
- net N$153: now also Q20.G2, R94.2; no longer R118.6, R33.2, U15.4
- net N$154: now also Q19.1, R23.6, R93.2; no longer R123.2, R44.2, U24.2
- net N$155: now also Q21.2, R23.4, R96.2; no longer R123.4, R45.2, U24.4
- net N$156: now also Q21.7, R99.1; no longer R124.2, R48.2, U27.2
- net N$157: now also Q22.G1, R99.2; no longer R124.4, R49.2, U27.4
- net N$158: now also Q21.5, R98.1; no longer R125.2, R52.2, U30.2
- net N$159: now also Q22.G2, R98.2; no longer R125.4, R53.2, U30.4
- net N$16: now also Q27.2, R110.4, R115.2; no longer R26.2, U12.7
- net N$160: now also Q21.1, R23.2, R97.2; no longer R128.2, R56.2, U33.2
- net N$161: now also Q23.2, R100.4, R101.2; no longer R128.4, R57.2, U33.4
- net N$162: now also Q23.7, R104.1; no longer R120.4, R60.2, U36.2
- net N$163: now also Q24.G1, R104.2; no longer R120.2, R61.2, U36.4
- net N$164: now also Q23.5, R103.1; no longer R120.8, R64.2, U39.2
- net N$165: now also Q24.G2, R103.2; no longer R120.6, R65.2, U39.4
- net N$166: now also Q23.1, R100.2, R102.2; no longer R131.2, R76.2, U48.2
- net N$167: now also C67.1, D4.C1, Q19.8; no longer R131.4, R77.2, U48.4
- net N$168: now also C69.1, D4.C2, Q21.8; no longer R130.2, R72.2, U45.2
- net N$169: now also C71.1, D4.C3, Q23.8; no longer R130.4, R73.2, U45.4
- net N$17: now also Q27.7, R118.1; no longer R27.2, U12.5
- net N$170: now also D4.A1, R24.7; no longer R129.2, R68.2, U42.2
- net N$171: now also D4.A3, R24.3; no longer R129.4, R69.2, U42.4
- net N$172: now also U5.13, U6.3; no longer U10.13, U13.3
- net N$173: now also C8.2; no longer C13.2
- net N$18: now also Q4.G1, R118.2; no longer Q1.4, R18.1
- net N$19: now also Q27.5, R117.1; no longer Q10.4, R67.1
- net N$2: now also R55.4; no longer R3.4
- net N$20: now also D8.A2, R29.5; no longer Q21.4, R26.1
- net N$21: now also Q4.G2, R117.2; no longer Q22.4, R27.1
- net N$22: now also Q27.1, R110.2, R116.2; no longer R30.2, U15.7
- net N$23: now also Q29.2, R119.4, R120.2; no longer R31.2, U15.5
- net N$24: now also Q29.7, R123.1; no longer Q3.4, R30.1
- net N$25: now also Q6.G1, R123.2; no longer Q14.4, R35.1
- net N$26: now also Q29.5, R122.1; no longer R34.2, U18.7
- net N$27: now also Q6.G2, R122.2; no longer R35.2, U18.5
- net N$28: now also Q29.1, R119.2, R121.2; no longer Q13.4, R34.1
- net N$29: now also C75.1, D8.C1, Q25.8; no longer Q16.4, R47.1
- net N$30: now also C77.1, D8.C2, Q27.8; no longer R38.2, U21.7
- net N$31: now also C79.1, D8.C3, Q29.8; no longer R39.2, U21.5
- net N$32: now also D8.A1, R29.7; no longer Q23.4, R38.1
- net N$33: now also D8.A3, R29.3; no longer Q24.4, R39.1
- net N$34: now also Q1.2, R3.8; no longer U24.7
- net N$35: now also Q1.7, R45.1; no longer R43.2, U24.5
- net N$36: now also D1.A2, R2.5; no longer Q5.4, R42.1
- net N$37: now also Q8.G1, R45.2; no longer Q18.4, R59.1
- net N$38: now also Q1.5, R44.1; no longer R46.2, U27.7
- net N$39: now also Q8.G2, R44.2; no longer R47.2, U27.5
- net N$4: now also R55.8; no longer R3.8
- net N$40: now also Q1.1, R3.6, R43.2; no longer Q15.4, R46.1
- net N$41: now also Q3.2, R3.4, R46.2; no longer Q20.4, R71.1
- net N$42: now also Q3.7, R49.1; no longer R50.2, U30.7
- net N$43: now also Q10.G1, R49.2; no longer R51.2, U30.5
- net N$44: now also Q3.5, R48.1; no longer Q25.4, R50.1
- net N$45: now also Q10.G2, R48.2; no longer J17.6, R88.2
- net N$46: now also Q3.1, R3.2, R47.2; no longer R54.2, U33.7
- net N$47: now also Q5.2, R50.2, R54.4; no longer R55.2, U33.5
- net N$48: now also Q5.7, R53.1; no longer Q7.4, R54.1
- net N$49: now also Q12.G1, R53.2; no longer Q26.4, R51.1
- net N$5: now also Q25.7, R114.1; no longer Q2.4, R19.1
- net N$50: now also Q5.5, R52.1; no longer R58.2, U36.7
- net N$51: now also Q12.G2, R52.2; no longer R59.2, U36.5
- net N$52: now also Q5.1, R51.2, R54.2; no longer Q17.4, R58.1
- net N$53: now also C38.1, D1.C1, Q1.8; no longer Q28.4, R63.1
- net N$54: now also C40.1, D1.C2, Q3.8; no longer R62.2, U39.7
- net N$55: now also C42.1, D1.C3, Q5.8; no longer R63.2, U39.5
- net N$56: now also D1.A1, R2.7; no longer Q27.4, R62.1
- net N$57: now also D1.A3, R2.3; no longer Q30.4, R75.1
- net N$58: now also Q13.2, R73.8, R74.2; no longer R66.2, U42.7
- net N$59: now also Q13.7, R77.1; no longer R67.2, U42.5
- net N$6: now also Q2.G1, R114.2; no longer R22.2, U9.7
- net N$60: now also D3.A2, R8.5; no longer Q9.4, R66.1
- net N$61: now also C22.1, R38.1, U10.3, U11.1, U11.3, U12.1, U12.3; no longer C1.1, R15.1, U4.1, U4.3, U5.1, U5.3, U8.3
- net N$62: now also Q14.G1, R77.2; no longer R70.2, U45.7
- net N$63: now also Q13.5, R76.1; no longer R71.2, U45.5
- net N$64: now also Q14.G2, R76.2; no longer Q19.4, R70.1
- net N$65: now also R71.2; no longer R9.2
- net N$66: now also Q13.1, R73.6, R75.2; no longer R74.2, U48.7
- net N$67: now also Q15.2, R73.4, R78.2; no longer R75.2, U48.5
- net N$68: now also Q15.7, R81.1; no longer Q29.4, R74.1
- net N$69: now also C19.2, D6.C, U9.6; no longer C43.2, D1.C, U3.6
- net N$7: now also Q25.5, R113.1; no longer R18.2, U6.7
- net N$70: now also R33.2; no longer R6.2
- net N$71: now also Q16.G1, R81.2; no longer J4.9, R6.4
- net N$72: now also R33.6; no longer R6.6
- net N$73: now also Q15.5, R80.1; no longer J5.8, R85.4
- net N$74: now also Q16.G2, R80.2; no longer J5.10, R85.8
- net N$75: now also J4.9, R33.4; no longer J5.9, R85.6
- net N$76: now also J5.8, R41.4; no longer J6.8, R86.2
- net N$77: now also J5.10, R41.8; no longer J6.10, R86.6
- net N$78: now also J5.9, R41.6; no longer J6.9, R86.4
- net N$79: now also J6.8, R10.2; no longer J7.8, R87.2
- net N$8: now also LED3.6, R106.1; no longer R23.2, U9.5
- net N$80: now also J6.10, R10.6; no longer J7.10, R87.6
- net N$81: now also J6.9, R10.4; no longer J7.9, R87.4
- net N$82: now also J7.8, R91.2; no longer J17.7, R88.4
- net N$83: now also J7.10, R91.6; no longer J17.8, R88.6
- net N$84: now also C2.1, U4.5; no longer C55.1, U20.5
- net N$85: now also J7.9, R91.4; no longer D4.C3, R1.1
- net N$86: now also J17.6, R56.2; no longer R117.6, R25.2, U9.4
- net N$87: now also J17.7, R56.4; no longer R117.8, R24.2, U9.2
- net N$88: now also R126.7; no longer R4.7
- net N$89: now also C23.1, R39.2, U11.5; no longer C34.1, R113.2, U4.5
- net N$9: now also LED3.5, R106.3; no longer Q4.4, R31.1
- net N$90: now also C24.1, R40.2, U12.5; no longer C31.1, R114.2, U5.5
- net N$91: now also R26.1, U2.50; no longer R80.1, U7.50
- net N$92: now also C12.2, R19.2, R20.1; no longer C18.2, R108.2, R93.1
- net N$93: now also J17.8, R56.6; no longer D4.C2, R1.5
- net N$96: now also Q17.2, R82.4, R83.2; no longer J11.1, S3.1, S3.4
- net N$97: now also R126.5; no longer R4.5
- net N$98: now also R126.3; no longer R4.3
- net N$99: now also R34.1, U9.4; no longer R5.1, U3.4
- net PROGB: now also R31.2; no longer R10.2
- net RADIO_INT: now also U2.16, U5.3; no longer U10.3, U7.16
- net RADIO_NCS: now also R15.1, U2.14, U5.7; no longer R116.1, U10.7, U7.14
- net RADIO_VDD: now also C57.1, C58.1, C59.1, C60.1, C62.1, U5.11, U5.14, U5.15, U5.18, U5.4, U5.9; no longer C11.1, C12.1, C6.1, C8.1, C9.1, U10.11, U10.14, U10.15, U10.18, U10.4, U10.9
- net SCK: now also R87.1, U2.21, U3.6, U5.1; no longer R2.1, U10.1, U2.6, U7.21
- net SRST: now also R22.1, U2.39; no longer R8.1, U7.39
- net SYSCLK: now also U2.62; no longer U7.62
- net TCK: now also R55.3, U2.53; no longer R3.3, U7.53
- net TMS: now also R55.1, U2.51; no longer R3.1, U7.51
- net TST: now also U2.40; no longer U7.40
- net VBUS: now also R17.1, R18.2, U2.52; no longer R107.1, R111.2, U7.52
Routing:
- net +1.8V: track 8.14 -> 80.1 mm, vias 5 -> 9
- net GND: track 418.8 -> 347.8 mm
- net LED_BF: track 0.00 -> 70.2 mm, vias 0 -> 4
- net LED_RY: track 69.2 -> 0.00 mm, vias 4 -> 0
- net LED_AN1: track 0.00 -> 68.8 mm, vias 0 -> 3
- net LED_AN2: track 0.00 -> 50.0 mm, vias 0 -> 2
- net LED_AE: track 0.00 -> 48.7 mm, vias 0 -> 2
- net LED_LR: track 47.4 -> 0.00 mm, vias 2 -> 0
- net LED_LY: track 45.5 -> 0.00 mm, vias 2 -> 0
- net LED_CG: track 0.00 -> 40.8 mm, vias 0 -> 2
- net LED_RR: track 40.6 -> 0.00 mm, vias 2 -> 0
- net LED_DDP: track 0.00 -> 39.1 mm, vias 0 -> 2
- net LED_RG: track 38.7 -> 0.00 mm, vias 2 -> 0
- net N$31: track 2.87 -> 35.5 mm, vias 0 -> 1
- net N$40: track 1.82 -> 29.8 mm, vias 0 -> 1
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- added copper zone on layer 2, net CHASSIS
- added copper zone on layer 1, net N$94
- added copper zone on layer 1, net VBATT
- removed copper zone on layer 16, net GND
- removed copper zone on layer 1, net N$103
- removed copper zone on layer 1, net N$96
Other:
- board text added: "Control 2014 Rev A"
- board text removed: "+"
- board text removed: "-"
- board text removed: "12V"
- board text removed: "3.3V"
- board text removed: "5V"
- board text removed: "ANT"
- board text removed: "BATTERY"
- board text removed: "Control 2011 Rev C"
- board text removed: "DISCHARGE"
- board text removed: "ENC3"
- board text removed: "ENC4"
- board text removed: "GND"
- board text removed: "ID"
- board text removed: "M3"
- board text removed: "M4"
- board text removed: "SPARE"
